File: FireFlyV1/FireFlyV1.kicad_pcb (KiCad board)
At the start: 2 copper layers, 64 x 26.2 mm, 59 parts, among them J1 Conn_01x03, J2 Conn_01x01_Pin, J3 Conn_01x01_Pin, SW1 TS-1187A-B-A-B, SW2 TS-1187A-B-A-B, U1 RP2040, U2 W25Q32JVSS, U3 AMS1117-3.3, U5 MCP6001T-I/OT, U7 PEC12R-4215F-S0024, X1 X322512MSB4SI

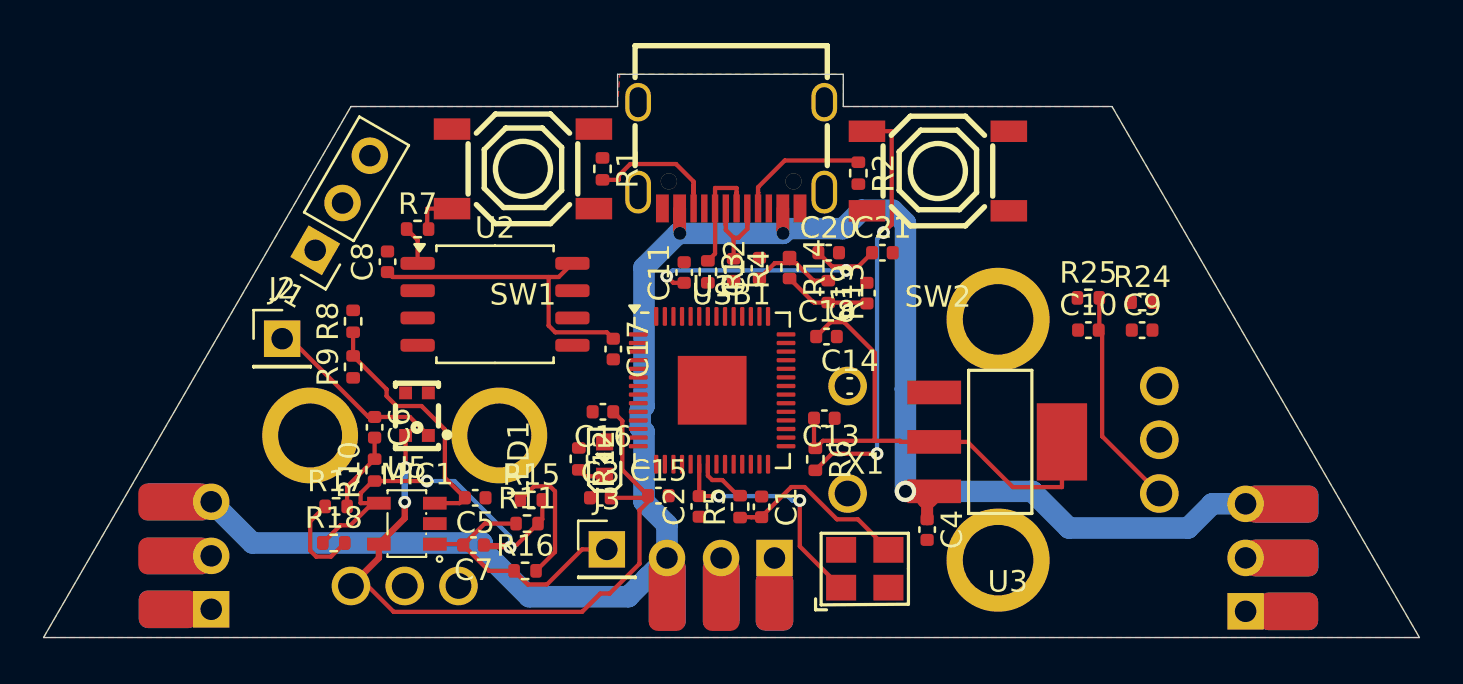
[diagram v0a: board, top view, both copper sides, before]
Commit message: First JLCPCB Order
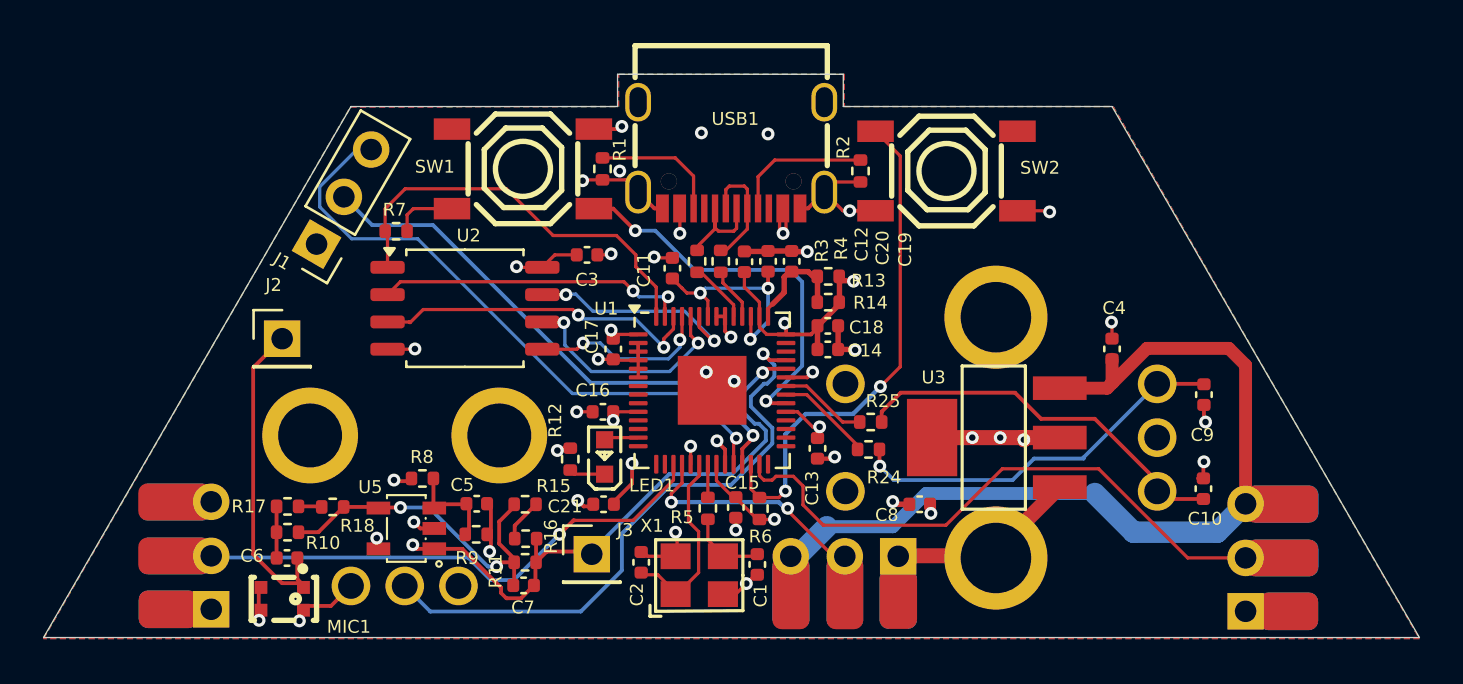
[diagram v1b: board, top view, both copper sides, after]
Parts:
- moved C8 27.2 mm to (223.8, 113.0), turned to 180 degrees
- moved C21 17.5 mm to (209.1, 113.0), turned to 180 degrees
- moved R24 14.5 mm to (221.4, 110.5)
- moved C4 12.0 mm to (232.7, 105.8), turned to 90 degrees
- moved R25 11.7 mm to (221.5, 109.2)
- moved C3 11.3 mm to (208.3, 101.4), turned to 180 degrees
- moved MIC1 10.6 mm to (194.1, 117.4), turned to -90 degrees
- moved R9 9.67 mm to (203.1, 114.4), turned to 180 degrees
- moved C10 9.11 mm to (236.9, 112.3), turned to -90 degrees
- moved R8 7.99 mm to (200.6, 111.8), turned to 180 degrees
- moved X1 7.71 mm to (213.5, 116.3)
- moved C6 7.32 mm to (194.3, 115.5), turned to 180 degrees
- moved LEDS2 5.76 mm to (220.3, 118.9)
- moved R10 4.98 mm to (194.3, 114.3), turned to 180 degrees
- moved C9 4.16 mm to (237.0, 107.9), turned to -90 degrees
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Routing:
- net BOARD_ID_0: track 6.00 -> 51.5 mm, vias 0 -> 30
- net 3V3: track 75.9 -> 36.0 mm, vias 2 -> 15
- net SWCLK: track 0.00 -> 29.3 mm, vias 0 -> 1
- net POT_ADC: track 0.00 -> 28.4 mm, vias 0 -> 1
- net SWDIO: track 0.00 -> 25.2 mm, vias 0 -> 1
- net LED_OUT_3: track 3.40 -> 27.6 mm
- net LED_OUT_1: track 3.85 -> 24.6 mm, vias 0 -> 1
- net /A: track 0.00 -> 19.3 mm, vias 0 -> 1
- net BUTTON: track 0.00 -> 18.4 mm, vias 0 -> 2
- net QSPI_SS: track 1.81 -> 19.3 mm
- net QSPI_SD2: track 0.00 -> 15.5 mm, vias 0 -> 2
- net MIC_ADC: track 12.3 -> 27.7 mm, vias 0 -> 2
- net QSPI_SP1: track 0.00 -> 14.6 mm, vias 0 -> 2
- net +5V: track 98.0 -> 110.7 mm, vias 3 -> 2
- net Net-(U1-VREG_VOUT): track 12.6 -> 24.4 mm, vias 2 -> 5
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- added copper zone on In1.Cu, net 3V3
- added copper zone on B.Cu, net BOARD_ID_0
- added copper zone on In2.Cu, net BOARD_ID_0
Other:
- copper layers 2 -> 4
- board text added: "FireFlyV1 @KylarLEDs"
